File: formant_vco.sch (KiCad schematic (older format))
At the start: 82 parts, among them J1 JACK_2P, J2 JACK_2P, J3 JACK_2P, J4 CONN_02X08, J5 JACK_2P, Q1 BC850, Q2 BC850, Q3 BC850, Q4 BC850, Q5 BC850, SW1 SWITCH_SPST, SW2 SWITCH_SPST, U1 REF102, U2 TL072, U3 CD4093, U4 TL072, U5 TL072, U6 LM3046, U7 TL072

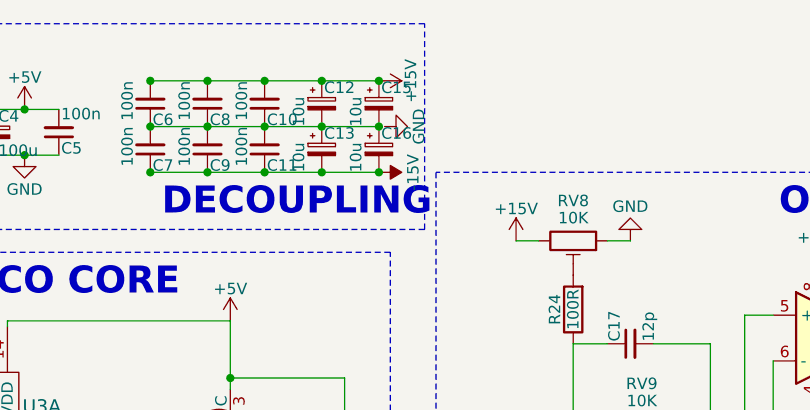
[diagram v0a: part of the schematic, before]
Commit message: Final routing, fab outputs
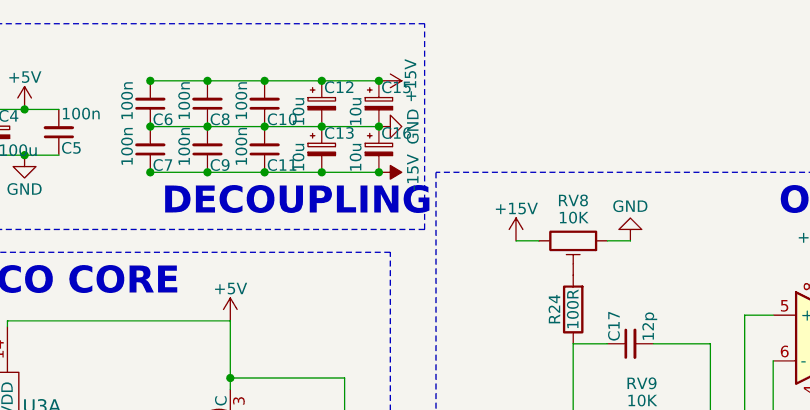
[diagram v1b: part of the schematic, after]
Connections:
- net GND: now also C10.1, C11.2, C12.2, C13.1, C15.2, C16.1, C6.1, C7.2, C8.1, C9.2
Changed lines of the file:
@@
 L GND #PWR035
 U 1 1 5965232A
-P 7775 1000
-F 0 "#PWR035" H 7775 750 50  0001 C CNN
-F 1 "GND" H 7775 850 50  0000 C CNN
-F 2 "" H 7775 1000 50  0001 C CNN
-F 3 "" H 7775 1000 50  0001 C CNN
-	1    7775 1000
+P 7750 1000
+F 0 "#PWR035" H 7750 750 50  0001 C CNN
+F 1 "GND" H 7750 850 50  0000 C CNN
+F 2 "" H 7750 1000 50  0001 C CNN
+F 3 "" H 7750 1000 50  0001 C CNN
+	1    7750 1000
 	0    -1   -1   0
 $EndComp
